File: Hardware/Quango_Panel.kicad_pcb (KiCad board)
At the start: 2 copper layers, 80.9 x 128.5 mm, 25 parts

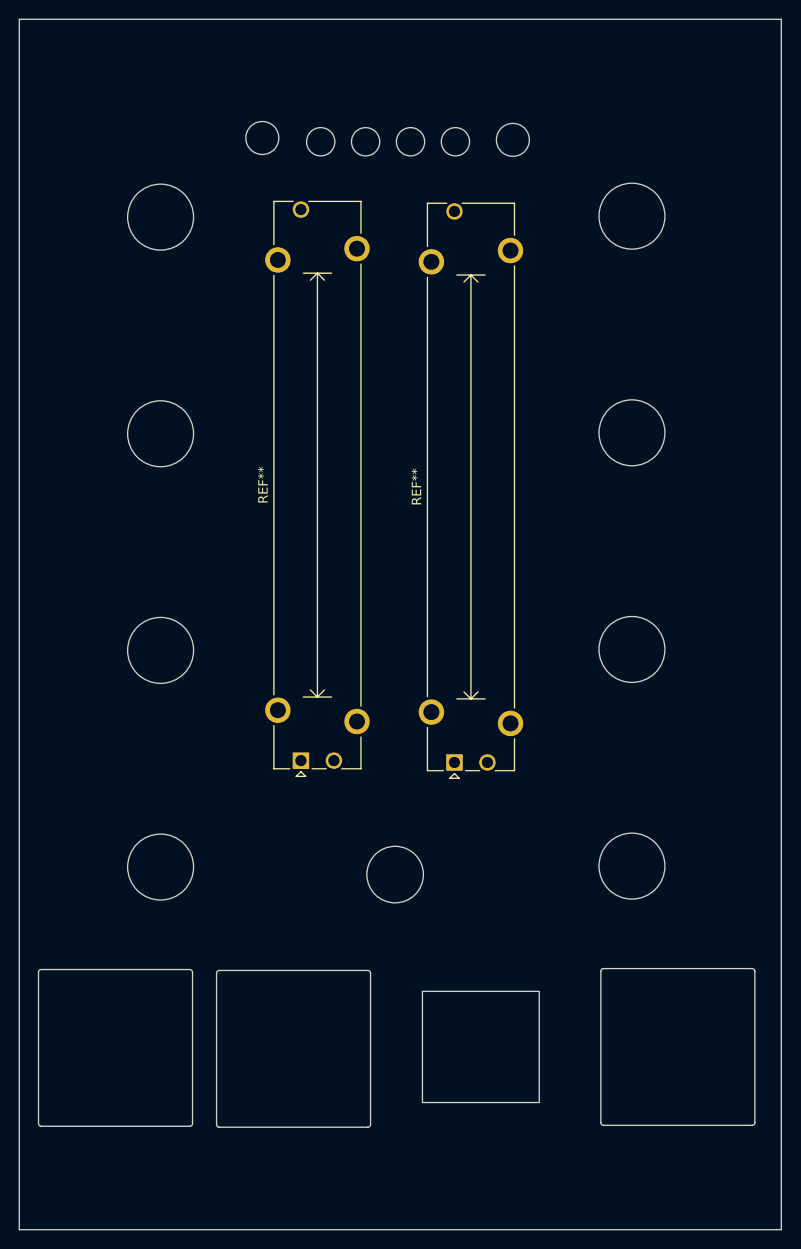
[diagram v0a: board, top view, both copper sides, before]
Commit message: More schematic updates
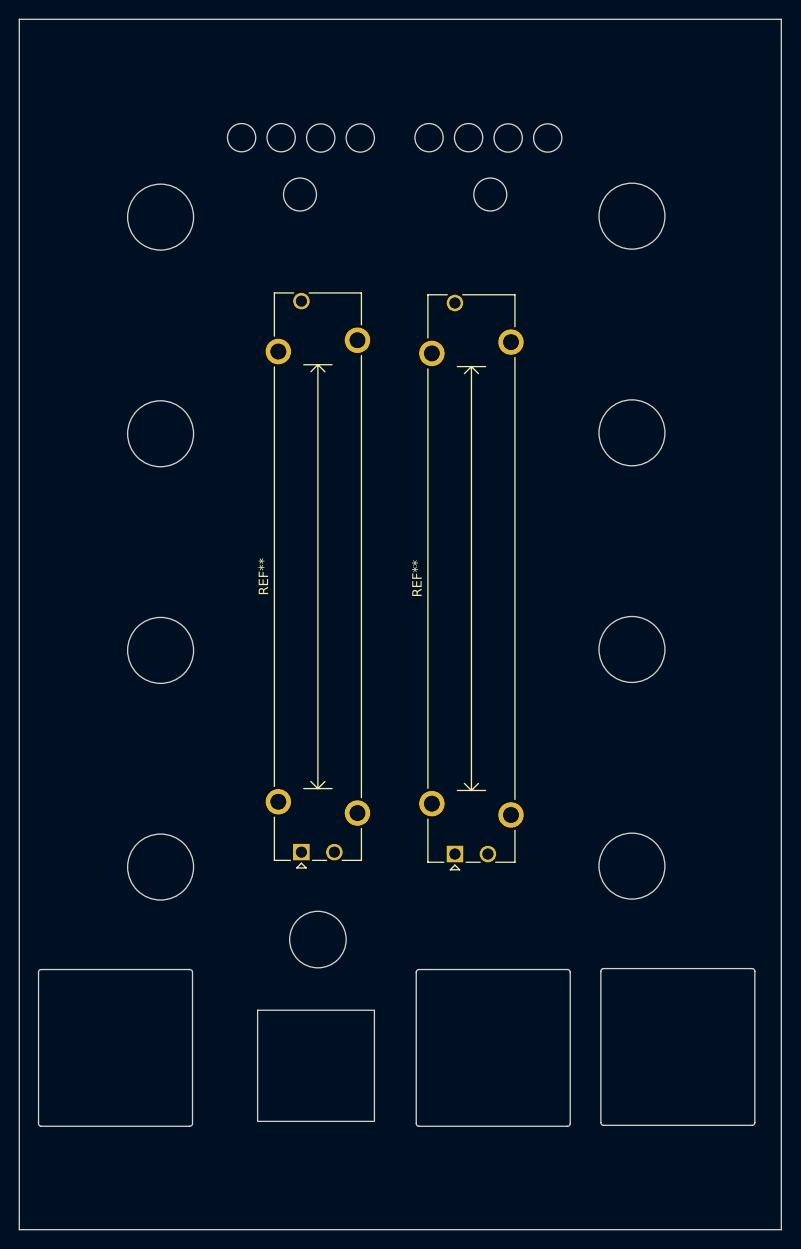
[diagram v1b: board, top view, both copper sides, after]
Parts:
- added Ref**: Subminiature_Switch, Custom_Footprints:LED_Hole_3mm, F.Cu at (106.1, 42.6)
- added Ref**: Subminiature_Switch, Custom_Footprints:LED_Hole_3mm, F.Cu at (77.8, 42.6)
- added Ref**: Subminiature_Switch, Custom_Footprints:LED_Hole_3mm, F.Cu at (86.2, 42.6)
- added Ref**: Subminiature_Switch, Custom_Footprints:LED_Hole_3mm, F.Cu at (97.7, 42.6)
- moved REF** 21.2 mm to (100.3, 139.2)
- moved USB** 17.6 mm to (81.5, 141.1)
- moved Ref** 10.7 mm to (81.7, 127.7)
- moved REF** 9.72 mm to (80.0, 118.4)
- moved REF** 9.72 mm to (96.2, 118.6)
- moved Ref** 8.41 mm to (73.6, 42.6), turned to 90 degrees
- moved RESET 7.21 mm to (79.8, 48.6)
- moved RESET 6.28 mm to (100.0, 48.6)
- moved Ref** 5.61 mm to (101.9, 42.6), turned to 90 degrees
- moved Ref** 4.78 mm to (82.0, 42.6), turned to 90 degrees
- moved Ref** 2.01 mm to (93.5, 42.6), turned to 90 degrees
